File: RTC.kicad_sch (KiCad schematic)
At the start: 7 parts, among them P16 CONN_4, U47 M6242, X1 RTC_OSC

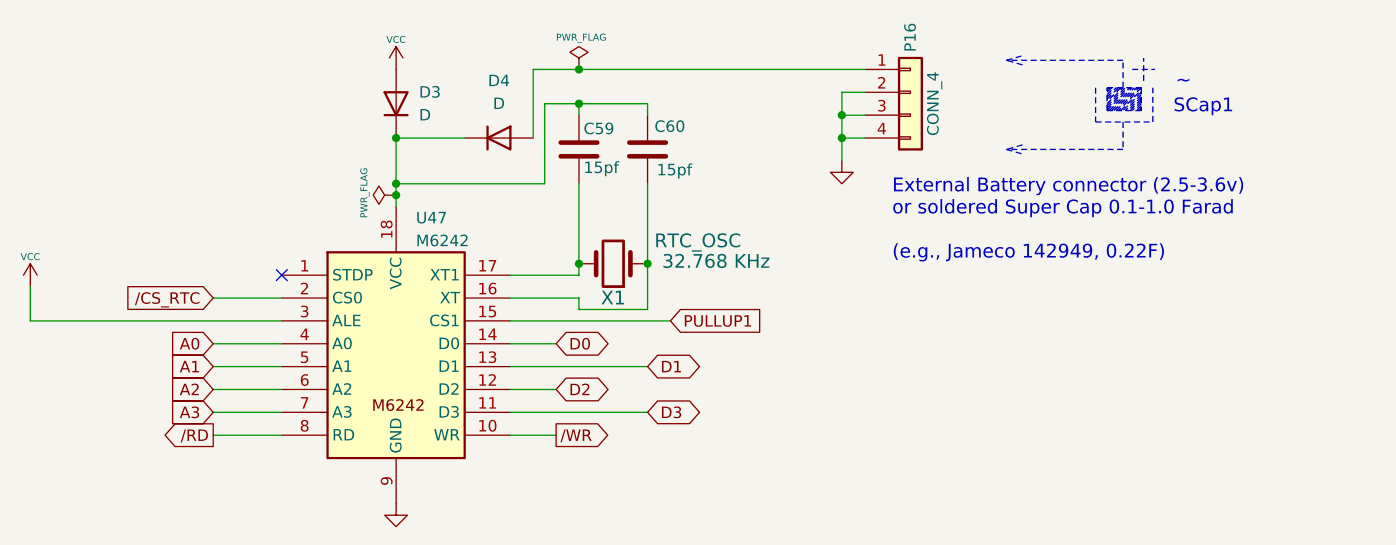
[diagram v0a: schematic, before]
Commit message: rev 1.0
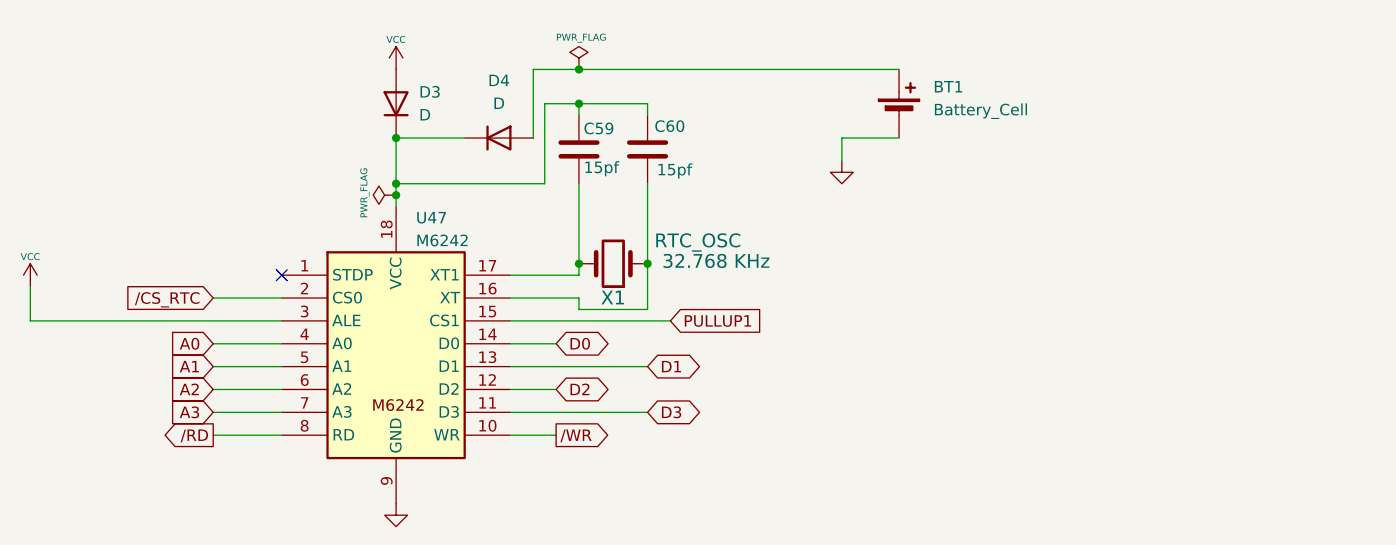
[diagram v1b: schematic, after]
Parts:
- removed P16: CONN_4, Custom:STD_DDW_PINHEAD_V_1x04, symbol Connector_Generic:Conn_01x04
- added BT1: Battery_Cell, Battery:BatteryHolder_MYOUNG_BS-07-A1BJ001_CR2032, symbol Device:Battery_Cell
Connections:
- net GND: now also BT1.2 (-)
- net at D4.2 (A): now also BT1.1 (+)
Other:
- note removed: "External Battery connector (2.5-3.6v) or soldered Super Cap 0.1-1.0 Farad (e.g., Jameco 142949, 0.22F)"
- note removed: "SCap1"
- note removed: "~"
